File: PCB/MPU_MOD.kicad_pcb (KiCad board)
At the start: 8 copper layers, 45 x 50 mm, 308 parts, among them J501 MEM2090-00-145-00-A_REVA, J701 FTSH-107-01-L-DV-K-A, J801 USB4215-03-A_REVA, J901 73412-0110, Q1 STL9P3LLH6, U1 IS21ES08GA-JQLI-TR, U201 STC3115IQT, U202 BQ25606RGER, U203 STPMIC1APQR, U3 BQ24298RTWR, U301 STM32MP157FABx, U401 MT41K256M16TW-107_P, U502 HSP051-4M10, U503 HSP051-4M10, U701 HSP051-4M10, U702 HSP051-4M10, U801 FUSB302BMPX, U802 HSP051-4M10, U901 LBEE5PK2AE-771, Y601 NX2012SA-32.768K, Y701 ECS-2520MVQ-240

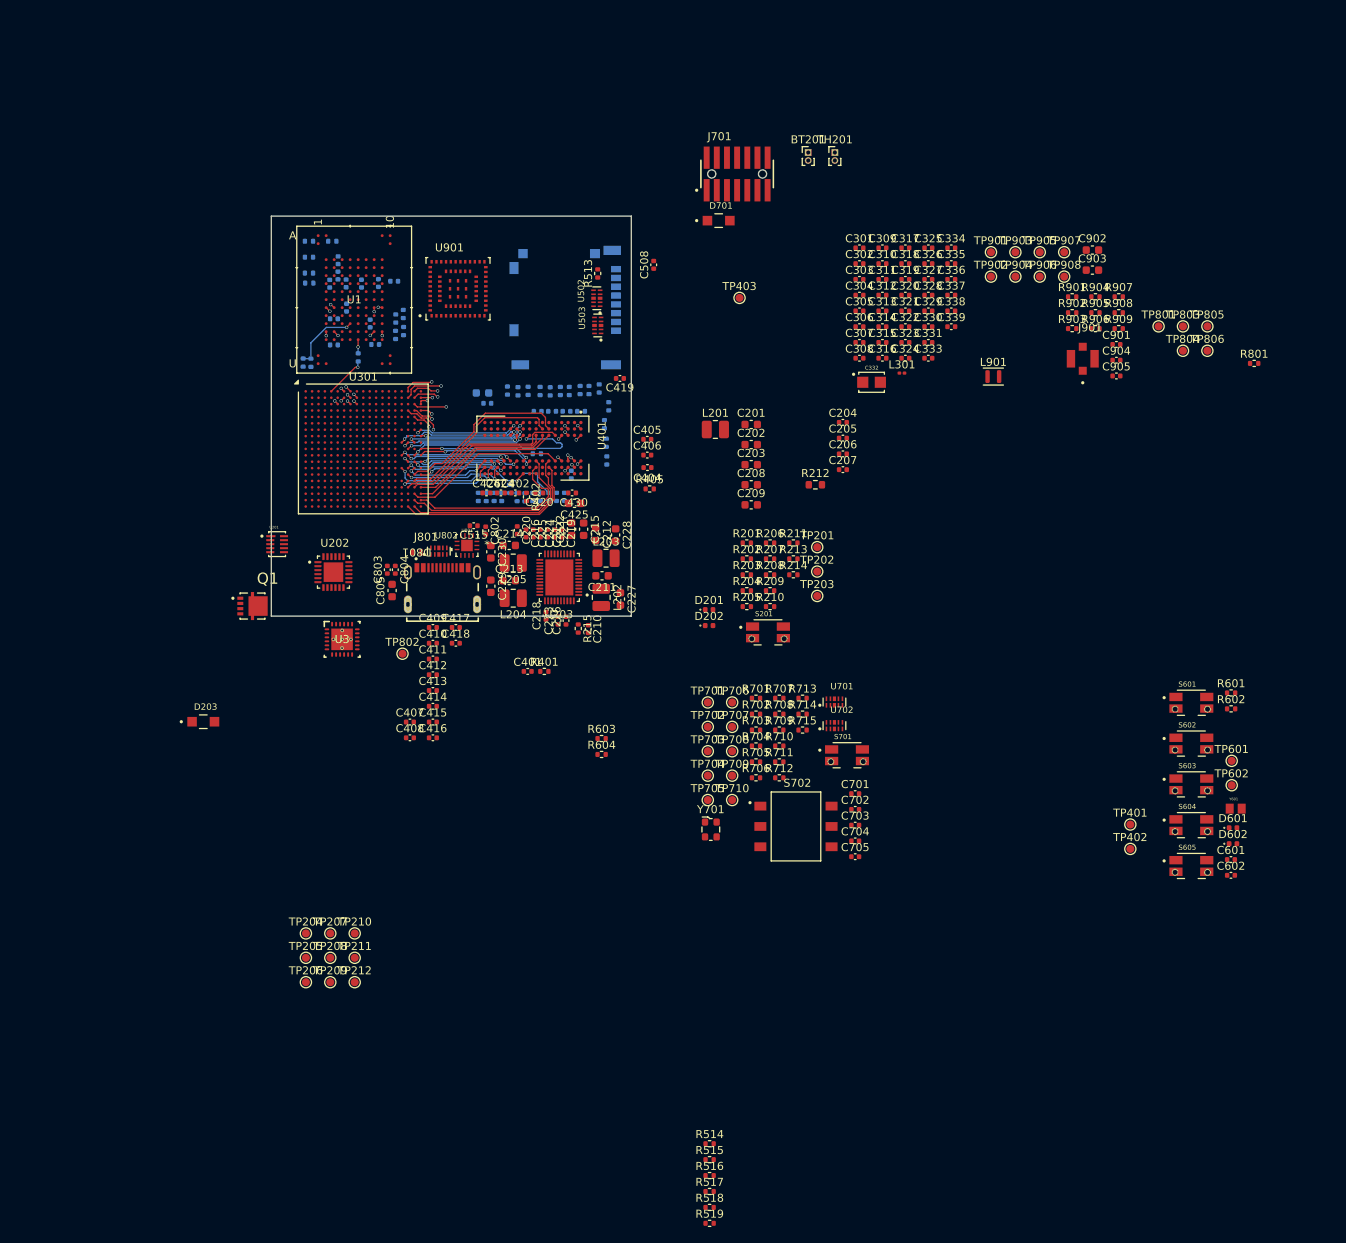
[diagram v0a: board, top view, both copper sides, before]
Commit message: PCB_UPDATE
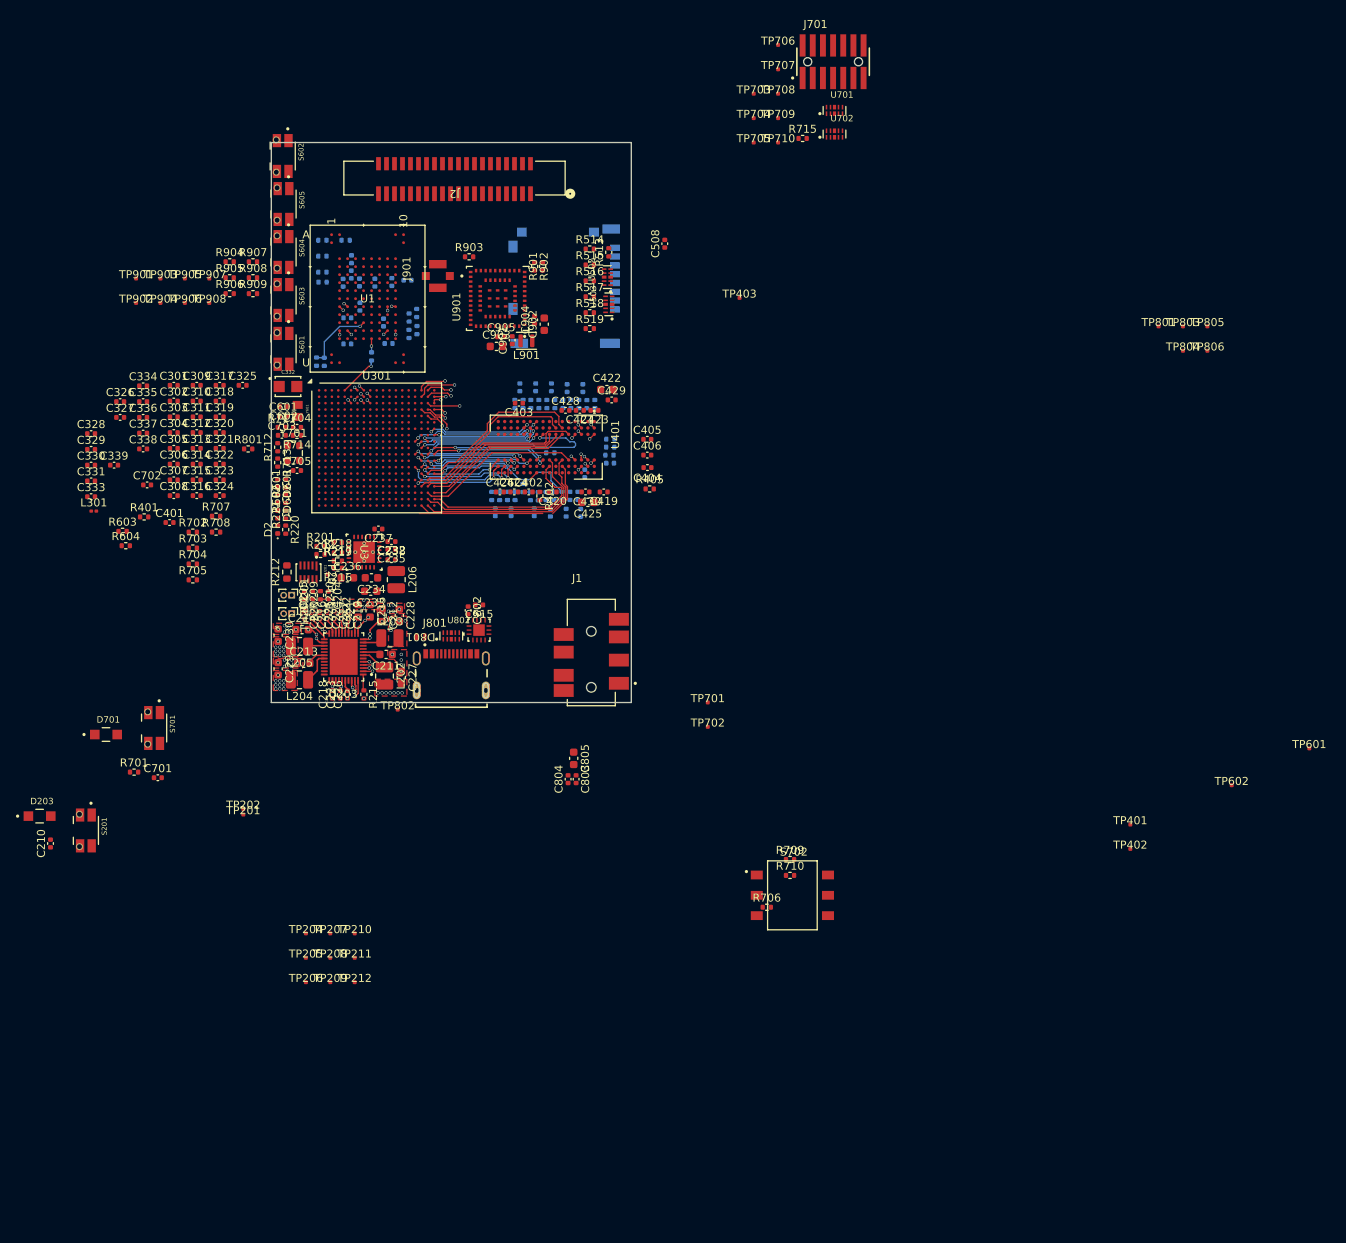
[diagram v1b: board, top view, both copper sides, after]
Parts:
- removed C201, C202, C203, C208, C209: 10uF, Capacitor_SMD:C_0603_1608Metric
- removed C206: 47nF, Capacitor_SMD:C_0402_1005Metric
- removed C207: 4.7uF, Capacitor_SMD:C_0402_1005Metric
- removed D201: LED_R, LED_SMD:LED_0402_1005Metric
- removed D202: LED_B, LED_SMD:LED_0402_1005Metric
- removed L201: 1uH, Inductor_SMD:L_1008_2520Metric
- removed Q1: STL9P3LLH6, lib:TRANS_STL9P3LLH6
- removed R203, R207: 0, Resistor_SMD:R_0402_1005Metric
- removed R204, R205: 2k2, Resistor_SMD:R_0402_1005Metric
- removed R206: 220, Resistor_SMD:R_0402_1005Metric
- removed R208: 10k, Resistor_SMD:R_0402_1005Metric
- removed R211: 240, Resistor_SMD:R_0402_1005Metric
- removed R213: 5k23, Resistor_SMD:R_0402_1005Metric
- removed R214: 30k1, Resistor_SMD:R_0402_1005Metric
- removed U202: BQ25606RGER, lib:QFN50P400X400X100-25N
- added C232: 47nF, Capacitor_SMD:C_0402_1005Metric, F.Cu at (83.5, 82.8)
- added C233: 10uF, Capacitor_SMD:C_0603_1608Metric, F.Cu at (80.9, 86.8)
- added C234: 10uF, Capacitor_SMD:C_0603_1608Metric, F.Cu at (81.0, 85.1)
- added C235: 4.7uF, Capacitor_SMD:C_0402_1005Metric, F.Cu at (83.5, 81.5)
- added C236: 10uF, Capacitor_SMD:C_0603_1608Metric, F.Cu at (78.0, 85.1)
- added C237: 1uF, Capacitor_SMD:C_0402_1005Metric, F.Cu at (81.9, 79.0)
- added C238: 8.2uF, Capacitor_SMD:C_0402_1005Metric, F.Cu at (83.5, 80.6)
- added D1: LED, LED_SMD:LED_0402_1005Metric, F.Cu at (69.3, 77.2)
- added D2: LED, LED_SMD:LED_0402_1005Metric, F.Cu at (69.3, 79.1)
- added J1: SJ3-35024K-SMT-TR, lib:SAMESKY_SJ3-35024K-SMT-TR, F.Cu at (112.0, 98.3)
- added J2: 2-1734248-0, lib:CONN_2-1734248-0_TYCO, F.Cu at (100.9, 37.1)
- added L206: 1uH, Inductor_SMD:L_1008_2520Metric, F.Cu at (84.1, 85.3)
- added R216: 5k25, Resistor_SMD:R_0402_1005Metric, F.Cu at (76.8, 83.9)
- added R217: 31k23, Resistor_SMD:R_0402_1005Metric, F.Cu at (76.8, 83.0)
- added R218: 317, Resistor_SMD:R_0402_1005Metric, F.Cu at (76.8, 82.0)
- added R219: 10k, Resistor_SMD:R_0402_1005Metric, F.Cu at (76.8, 80.7)
- added R220: 1k, Resistor_SMD:R_0402_1005Metric, F.Cu at (70.3, 79.1)
- added R221: 1k, Resistor_SMD:R_0402_1005Metric, F.Cu at (70.3, 77.2)
- C403, C421, C422, C423, C428, C429: moved to F.Cu
- C407, C408, C409, C410, C411, C412, C413, C414, C415, C416, C417, C418: moved to B.Cu
- TP201, TP202, TP203, TP204, TP205, TP206, TP207, TP208, TP209, TP210, TP211, TP212, TP401, TP402, TP403, TP601, TP602, TP701, TP702, TP703, TP704, TP705, TP706, TP707, TP708, TP709, TP710, TP801, TP802, TP803, TP804, TP805, TP806, TP901, TP902, TP903, TP904, TP905, TP906, TP907, TP908: footprint TestPoint:TestPoint_Pad_D1.0mm -> Library:TP_0.5mm
- moved S605 140.4 mm to (70.0, 38.4), turned to -90 degrees
- moved S602 135.3 mm to (69.9, 32.4), turned to -90 degrees
- moved S604 134.2 mm to (70.0, 44.4), turned to -90 degrees
- moved C602 132.1 mm to (70.0, 63.7), turned to 180 degrees
- moved C601 130.8 mm to (70.0, 64.9)
- moved S603 128.6 mm to (70.0, 50.4), turned to -90 degrees
- moved Y601 127.4 mm to (71.8, 64.2), turned to -90 degrees
- moved D602 127.0 mm to (69.3, 75.2), turned to -90 degrees
- moved D601 126.9 mm to (69.3, 73.3), turned to -90 degrees
- moved R801 126.2 mm to (65.6, 69.0)
- moved S601 121.8 mm to (70.0, 56.5), turned to -90 degrees
- moved R602 121.1 mm to (70.3, 75.2), turned to 90 degrees
- moved R601 121.0 mm to (70.3, 73.3), turned to 90 degrees
- moved R514 112.8 mm to (108.3, 44.0)
- moved R515 112.8 mm to (108.3, 46.0)
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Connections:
- R201 pad 2: +BATT -> VDD
- R202 pad 2: +BATT -> VDD
- TP201 pad 1: CHRG_NPG -> Net-(U3-STAT)
- TP202 pad 1: CHRG_STAT -> Net-(U3-PG_N)
- U3 pad 1: unconnected-(U3-VBUS-Pad1) -> V_USB
- U3 pad 10: unconnected-(U3-ILIM-Pad10) -> Net-(U3-ILIM)
- U3 pad 11: unconnected-(U3-TS-Pad11) -> /PWR/BATT_T
- U3 pad 13: unconnected-(U3-BAT-Pad13) -> +BATT
- U3 pad 14: unconnected-(U3-BAT-Pad14) -> +BATT
- U3 pad 15: unconnected-(U3-SYS-Pad15) -> VIN
- U3 pad 16: unconnected-(U3-SYS-Pad16) -> VIN
- U3 pad 17: unconnected-(U3-PGND-Pad17) -> GND
- U3 pad 18: unconnected-(U3-PGND-Pad18) -> GND
- U3 pad 19: unconnected-(U3-SW-Pad19) -> Net-(C232-Pad1)
- U3 pad 2: unconnected-(U3-PSEL-Pad2) -> CHRG_PSEL
- U3 pad 20: unconnected-(U3-SW-Pad20) -> Net-(C232-Pad1)
- U3 pad 21: unconnected-(U3-BTST-Pad21) -> Net-(U3-BTST)
- U3 pad 22: unconnected-(U3-REGN-Pad22) -> /PWR/REGN
- U3 pad 23: unconnected-(U3-PMID-Pad23) -> Net-(U3-PMID)
- U3 pad 24: unconnected-(U3-VBUS-Pad24) -> V_USB
- U3 pad 25: unconnected-(U3-PAD-Pad25) -> GND
- U3 pad 3: unconnected-(U3-PG_N-Pad3) -> Net-(U3-PG_N)
- U3 pad 4: unconnected-(U3-STAT-Pad4) -> Net-(U3-STAT)
- U3 pad 5: unconnected-(U3-SCL-Pad5) -> SYS_I2C4_SCL
- U3 pad 6: unconnected-(U3-SDA-Pad6) -> SYS_I2C4_SDA
- U3 pad 7: unconnected-(U3-INT-Pad7) -> CHRG_INT
- U3 pad 8: unconnected-(U3-OTG-Pad8) -> CHRG_OTG_ON
- U3 pad 9: unconnected-(U3-CE_N-Pad9) -> GND
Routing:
- net VIN: track 0.00 -> 14.4 mm, vias 0 -> 9
- net Net-(U203-LDO1OUT): track 0.00 -> 3.99 mm, vias 0 -> 1
- net Net-(U203-VLX3): track 0.00 -> 3.90 mm
- net Net-(U203-VLX1): track 0.00 -> 3.69 mm
- net 3V3: track 0.00 -> 3.09 mm, vias 0 -> 13
- net Net-(U203-VLX2): track 0.00 -> 2.94 mm
- net Net-(U203-LDO6OUT): track 0.00 -> 2.79 mm, vias 0 -> 1
- net VDD_DDR: track 0.00 -> 2.59 mm, vias 0 -> 8
- net VDDA: track 0.00 -> 2.28 mm, vias 0 -> 1
- net PWR_ON: track 0.00 -> 2.16 mm, vias 0 -> 1
- net VTT_DDR: track 0.00 -> 2.13 mm, vias 0 -> 2
- net Net-(U203-LDO2OUT): track 0.00 -> 2.06 mm, vias 0 -> 1
- net Net-(U203-VLX4): track 0.00 -> 2.05 mm
- net Net-(U203-~{RST}): track 0.00 -> 2.02 mm
- net VREF_DDR: track 0.00 -> 1.82 mm, vias 0 -> 1
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- added copper zone on F.Cu, net 3V3
- added copper zone on F.Cu, net GND
- added copper zone on F.Cu, net VDD
- added copper zone on F.Cu, net VDD_CORE
- added copper zone on F.Cu, net VDD_DDR
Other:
- board size 45 x 50 mm -> 45 x 70 mm
